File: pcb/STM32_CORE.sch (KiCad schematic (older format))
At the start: 31 parts, among them J6 Conn_01x14, J7 Conn_01x12, J8 Conn_01x12, SW1 SW_Push, U3 STM32F103C8T6, U4 AMS1117-3.3, Y1 O8M, Y2 O32.768K

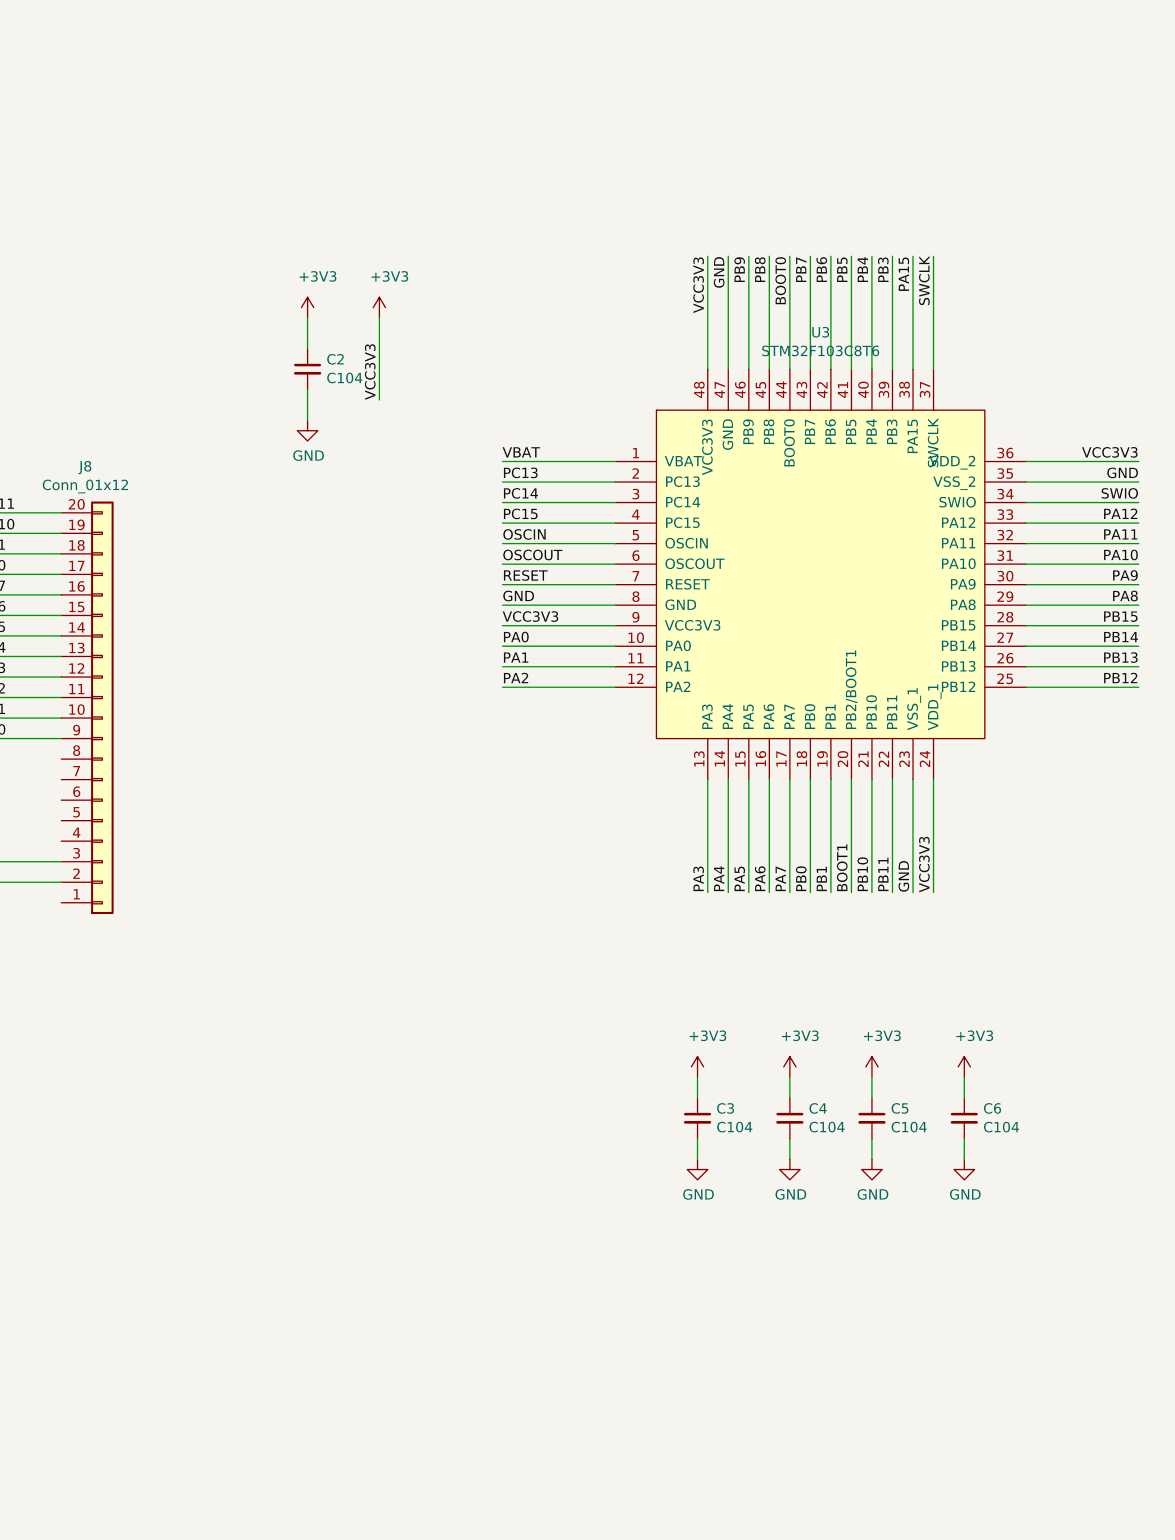
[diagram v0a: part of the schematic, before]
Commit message: update,
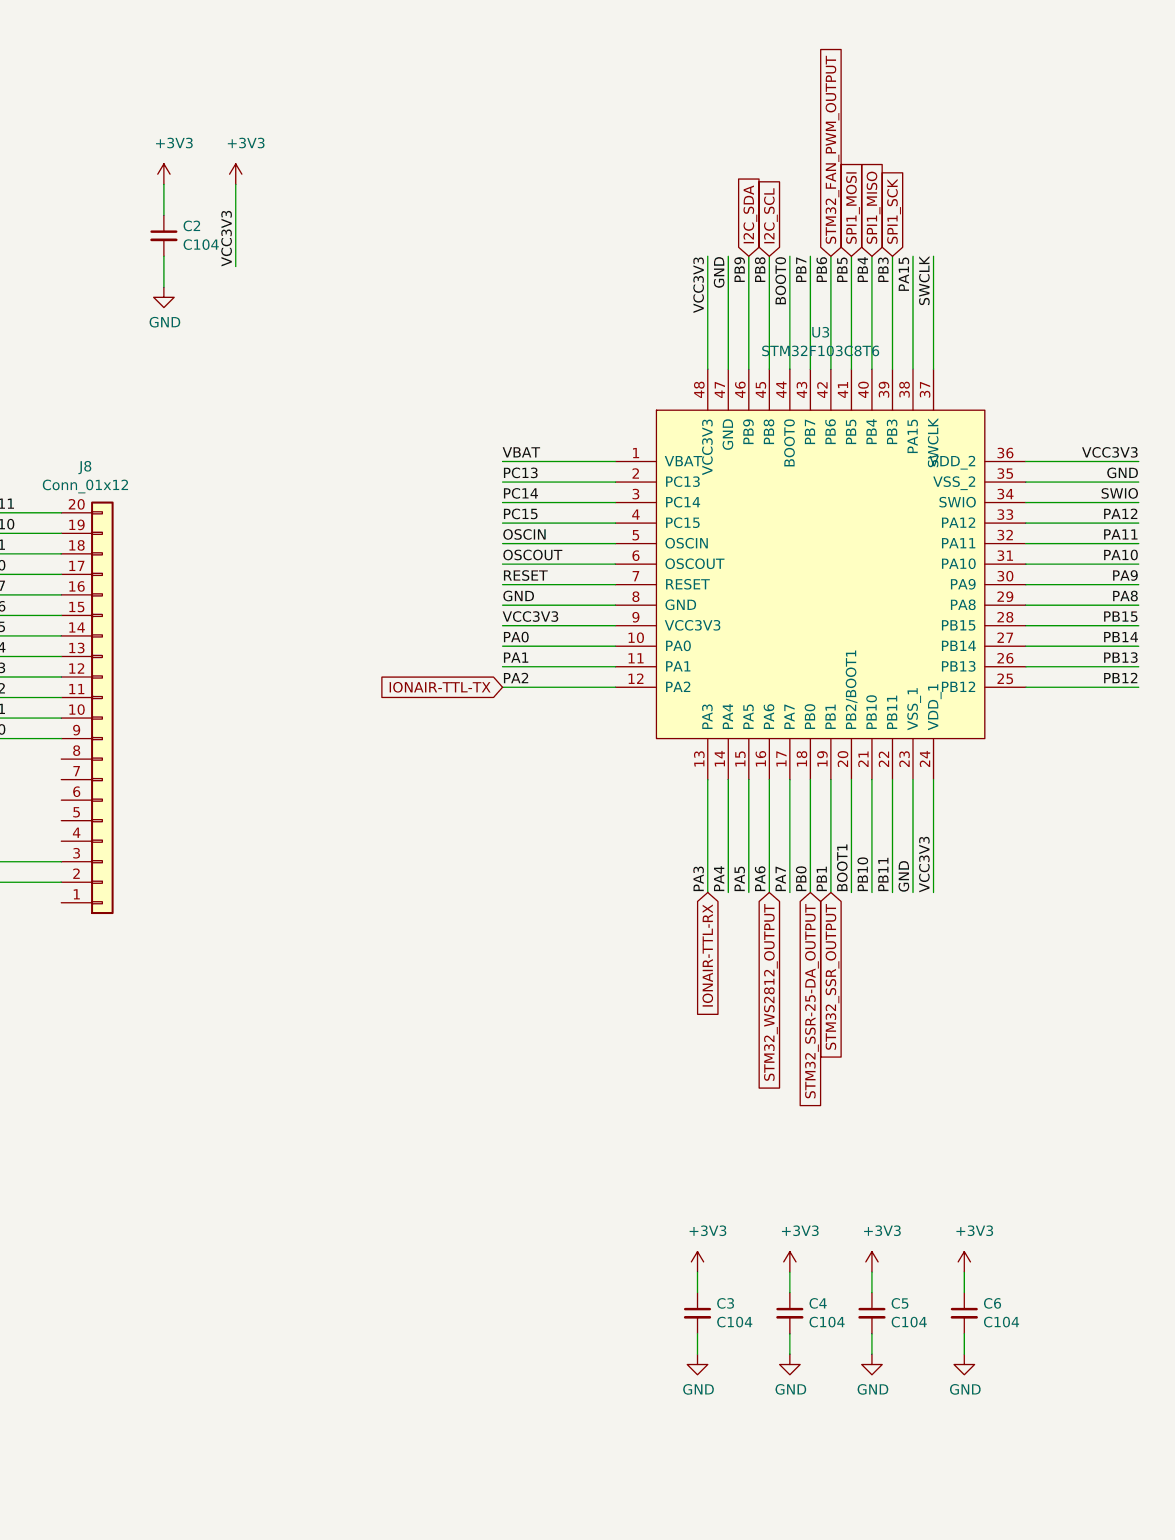
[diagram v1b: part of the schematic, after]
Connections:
- net PA2 renamed IONAIR-TTL-TX
- net PA3 renamed IONAIR-TTL-RX
- net PA6 renamed STM32_WS2812_OUTPUT
- net PB0 renamed STM32_SSR-25-DA_OUTPUT
- net PB1 renamed STM32_SSR_OUTPUT
- net PB3 renamed SPI1_SCK
- net PB4 renamed SPI1_MISO
- net PB5 renamed SPI1_MOSI
- net PB6 renamed STM32_FAN_PWM_OUTPUT
- net PB8 renamed I2C_SCL
- net PB9 renamed I2C_SDA
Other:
- moved on the sheet: C2, C3, C4, C5, C6
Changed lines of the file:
@@
 L taobao-c:C104 C3
 U 1 1 5BCBC4D6
-P 7850 5850
-F 0 "C3" H 7942 5896 50  0000 L CNN
-F 1 "C104" H 7942 5805 50  0000 L CNN
-F 2 "Capacitor_SMD:C_0603_1608Metric_Pad1.05x0.95mm_HandSolder" H 7850 5850 50  0001 C CNN
-F 3 "~" H 7850 5850 50  0001 C CNN
-	1    7850 5850
-	1    0    0    -1
-$EndComp
-Wire Wire Line
-	7850 5650 7850 5750
+P 7850 6800
+F 0 "C3" H 7942 6846 50  0000 L CNN
+F 1 "C104" H 7942 6755 50  0000 L CNN
+F 2 "Capacitor_SMD:C_0603_1608Metric_Pad1.05x0.95mm_HandSolder" H 7850 6800 50  0001 C CNN
+F 3 "~" H 7850 6800 50  0001 C CNN
+	1    7850 6800
+	1    0    0    -1
+$EndComp
+Wire Wire Line
+	7850 6600 7850 6700
 $Comp
 L power:GND #PWR026
 U 1 1 5BCBCE91
-P 7850 6050
-F 0 "#PWR026" H 7850 5800 50  0001 C CNN
-F 1 "GND" H 7855 5877 50  0000 C CNN
-F 2 "" H 7850 6050 50  0001 C CNN
-F 3 "" H 7850 6050 50  0001 C CNN
-	1    7850 6050
-	1    0    0    -1
-$EndComp
-Wire Wire Line
-	7850 5950 7850 6050
+P 7850 7000
+F 0 "#PWR026" H 7850 6750 50  0001 C CNN
+F 1 "GND" H 7855 6827 50  0000 C CNN
+F 2 "" H 7850 7000 50  0001 C CNN
+F 3 "" H 7850 7000 50  0001 C CNN
+	1    7850 7000
+	1    0    0    -1
+$EndComp
+Wire Wire Line
+	7850 6900 7850 7000
 $Comp
 L taobao-c:C104 C4
 U 1 1 5BCBD860
-P 8300 5850
-F 0 "C4" H 8392 5896 50  0000 L CNN
-F 1 "C104" H 8392 5805 50  0000 L CNN
-F 2 "Capacitor_SMD:C_0603_1608Metric_Pad1.05x0.95mm_HandSolder" H 8300 5850 50  0001 C CNN
-F 3 "~" H 8300 5850 50  0001 C CNN
-	1    8300 5850
-	1    0    0    -1
-$EndComp
-Wire Wire Line
-	8300 5650 8300 5750
+P 8300 6800
+F 0 "C4" H 8392 6846 50  0000 L CNN
+F 1 "C104" H 8392 6755 50  0000 L CNN
+F 2 "Capacitor_SMD:C_0603_1608Metric_Pad1.05x0.95mm_HandSolder" H 8300 6800 50  0001 C CNN
+F 3 "~" H 8300 6800 50  0001 C CNN
+	1    8300 6800
+	1    0    0    -1
+$EndComp
+Wire Wire Line
+	8300 6600 8300 6700
 $Comp
 L power:GND #PWR028
 U 1 1 5BCBD867
-P 8300 6050
-F 0 "#PWR028" H 8300 5800 50  0001 C CNN
-F 1 "GND" H 8305 5877 50  0000 C CNN
-F 2 "" H 8300 6050 50  0001 C CNN
-F 3 "" H 8300 6050 50  0001 C CNN
-	1    8300 6050
-	1    0    0    -1
-$EndComp
-Wire Wire Line
-	8300 5950 8300 6050
+P 8300 7000
+F 0 "#PWR028" H 8300 6750 50  0001 C CNN
+F 1 "GND" H 8305 6827 50  0000 C CNN
+F 2 "" H 8300 7000 50  0001 C CNN
+F 3 "" H 8300 7000 50  0001 C CNN
+	1    8300 7000
+	1    0    0    -1
+$EndComp
+Wire Wire Line
+	8300 6900 8300 7000
 $Comp
 L taobao-c:C104 C5
 U 1 1 5BCBE2F2
-P 8700 5850
-F 0 "C5" H 8792 5896 50  0000 L CNN
-F 1 "C104" H 8792 5805 50  0000 L CNN
-F 2 "Capacitor_SMD:C_0603_1608Metric_Pad1.05x0.95mm_HandSolder" H 8700 5850 50  0001 C CNN
-F 3 "~" H 8700 5850 50  0001 C CNN
-	1    8700 5850
-	1    0    0    -1
-$EndComp
-Wire Wire Line
-	8700 5650 8700 5750
+P 8700 6800
+F 0 "C5" H 8792 6846 50  0000 L CNN
+F 1 "C104" H 8792 6755 50  0000 L CNN
+F 2 "Capacitor_SMD:C_0603_1608Metric_Pad1.05x0.95mm_HandSolder" H 8700 6800 50  0001 C CNN
+F 3 "~" H 8700 6800 50  0001 C CNN
+	1    8700 6800
+	1    0    0    -1
+$EndComp
+Wire Wire Line
+	8700 6600 8700 6700
 $Comp
 L power:GND #PWR030
 U 1 1 5BCBE2F9
-P 8700 6050
-F 0 "#PWR030" H 8700 5800 50  0001 C CNN
-F 1 "GND" H 8705 5877 50  0000 C CNN
-F 2 "" H 8700 6050 50  0001 C CNN
-F 3 "" H 8700 6050 50  0001 C CNN
-	1    8700 6050
-	1    0    0    -1
-$EndComp
-Wire Wire Line
-	8700 5950 8700 6050
+P 8700 7000
+F 0 "#PWR030" H 8700 6750 50  0001 C CNN
+F 1 "GND" H 8705 6827 50  0000 C CNN
+F 2 "" H 8700 7000 50  0001 C CNN
+F 3 "" H 8700 7000 50  0001 C CNN
+	1    8700 7000
+	1    0    0    -1
+$EndComp
+Wire Wire Line
+	8700 6900 8700 7000
 $Comp
 L taobao-c:C104 C6
 U 1 1 5BCBE306
-P 9150 5850
-F 0 "C6" H 9242 5896 50  0000 L CNN
-F 1 "C104" H 9242 5805 50  0000 L CNN
-F 2 "Capacitor_SMD:C_0603_1608Metric_Pad1.05x0.95mm_HandSolder" H 9150 5850 50  0001 C CNN
-F 3 "~" H 9150 5850 50  0001 C CNN
-	1    9150 5850
-	1    0    0    -1
-$EndComp
-Wire Wire Line
-	9150 5650 9150 5750
+P 9150 6800
+F 0 "C6" H 9242 6846 50  0000 L CNN
+F 1 "C104" H 9242 6755 50  0000 L CNN
+F 2 "Capacitor_SMD:C_0603_1608Metric_Pad1.05x0.95mm_HandSolder" H 9150 6800 50  0001 C CNN
+F 3 "~" H 9150 6800 50  0001 C CNN
+	1    9150 6800
+	1    0    0    -1
+$EndComp
+Wire Wire Line
+	9150 6600 9150 6700
 $Comp
 L power:GND #PWR032
 U 1 1 5BCBE30D
-P 9150 6050
-F 0 "#PWR032" H 9150 5800 50  0001 C CNN
-F 1 "GND" H 9155 5877 50  0000 C CNN
-F 2 "" H 9150 6050 50  0001 C CNN
-F 3 "" H 9150 6050 50  0001 C CNN
-	1    9150 6050
-	1    0    0    -1
-$EndComp
-Wire Wire Line
-	9150 5950 9150 6050
+P 9150 7000
+F 0 "#PWR032" H 9150 6750 50  0001 C CNN
+F 1 "GND" H 9155 6827 50  0000 C CNN
+F 2 "" H 9150 7000 50  0001 C CNN
+F 3 "" H 9150 7000 50  0001 C CNN
+	1    9150 7000
+	1    0    0    -1
+$EndComp
+Wire Wire Line
+	9150 6900 9150 7000
 $Comp
 L taobao-osc:O32.768K Y2
@@
 L taobao-c:C104 C2
 U 1 1 5BD956B7
-P 5950 2200
-F 0 "C2" H 6042 2246 50  0000 L CNN
-F 1 "C104" H 6042 2155 50  0000 L CNN
-F 2 "Capacitor_SMD:C_0603_1608Metric_Pad1.05x0.95mm_HandSolder" H 5950 2200 50  0001 C CNN
-F 3 "~" H 5950 2200 50  0001 C CNN
-F 4 "near SWD" H 5950 2200 50  0001 C CNN "Field4"
-	1    5950 2200
+P 5250 1550
+F 0 "C2" H 5342 1596 50  0000 L CNN
+F 1 "C104" H 5342 1505 50  0000 L CNN
+F 2 "Capacitor_SMD:C_0603_1608Metric_Pad1.05x0.95mm_HandSolder" H 5250 1550 50  0001 C CNN
+F 3 "~" H 5250 1550 50  0001 C CNN
+F 4 "near SWD" H 5250 1550 50  0001 C CNN "Field4"
+	1    5250 1550
 	1    0    0    -1
 $EndComp
@@
 L power:GND #PWR023
 U 1 1 5BD957D4
-P 5950 2450
-F 0 "#PWR023" H 5950 2200 50  0001 C CNN
-F 1 "GND" H 5955 2277 50  0000 C CNN
-F 2 "" H 5950 2450 50  0001 C CNN
-F 3 "" H 5950 2450 50  0001 C CNN
-	1    5950 2450
-	1    0    0    -1
-$EndComp
-Wire Wire Line
-	5950 2300 5950 2450
-Wire Wire Line
-	5950 1950 5950 2100
+P 5250 1800
+F 0 "#PWR023" H 5250 1550 50  0001 C CNN
+F 1 "GND" H 5255 1627 50  0000 C CNN
+F 2 "" H 5250 1800 50  0001 C CNN
+F 3 "" H 5250 1800 50  0001 C CNN
+	1    5250 1800
+	1    0    0    -1
+$EndComp
+Wire Wire Line
+	5250 1650 5250 1800
+Wire Wire Line
+	5250 1300 5250 1450
 Text Label 2350 2600 2    50   ~ 0
 SWIO
@@
 	1    0    0    1
 $EndComp
-Text Label 6300 2350 1    50   ~ 0
+Text Label 5600 1700 1    50   ~ 0
 VCC3V3
 Wire Wire Line
-	6300 1950 6300 2350
+	5600 1300 5600 1700
 $Comp
 L Device:Jumper_NO_Small JP1
@@
 L power:+3V3 #PWR024
 U 1 1 5BCAD5BF
-P 6300 1950
-F 0 "#PWR024" H 6300 1800 50  0001 C CNN
-F 1 "+3V3" H 6350 2150 50  0000 C CNN
-F 2 "" H 6300 1950 50  0001 C CNN
-F 3 "" H 6300 1950 50  0001 C CNN
-	1    6300 1950
+P 5600 1300
+F 0 "#PWR024" H 5600 1150 50  0001 C CNN
+F 1 "+3V3" H 5650 1500 50  0000 C CNN
+F 2 "" H 5600 1300 50  0001 C CNN
+F 3 "" H 5600 1300 50  0001 C CNN
+	1    5600 1300
 	1    0    0    -1
 $EndComp
@@
 L power:+3V3 #PWR025
 U 1 1 5BCBE3DE
-P 7850 5650
-F 0 "#PWR025" H 7850 5500 50  0001 C CNN
-F 1 "+3V3" H 7900 5850 50  0000 C CNN
-F 2 "" H 7850 5650 50  0001 C CNN
-F 3 "" H 7850 5650 50  0001 C CNN
-	1    7850 5650
+P 7850 6600
+F 0 "#PWR025" H 7850 6450 50  0001 C CNN
+F 1 "+3V3" H 7900 6800 50  0000 C CNN
+F 2 "" H 7850 6600 50  0001 C CNN
+F 3 "" H 7850 6600 50  0001 C CNN
+	1    7850 6600
 	1    0    0    -1
 $EndComp
@@
 L power:+3V3 #PWR027
 U 1 1 5BCE7C1D
-P 8300 5650
-F 0 "#PWR027" H 8300 5500 50  0001 C CNN
-F 1 "+3V3" H 8350 5850 50  0000 C CNN
-F 2 "" H 8300 5650 50  0001 C CNN
-F 3 "" H 8300 5650 50  0001 C CNN
-	1    8300 5650
+P 8300 6600
+F 0 "#PWR027" H 8300 6450 50  0001 C CNN
+F 1 "+3V3" H 8350 6800 50  0000 C CNN
+F 2 "" H 8300 6600 50  0001 C CNN
+F 3 "" H 8300 6600 50  0001 C CNN
+	1    8300 6600
 	1    0    0    -1
 $EndComp
@@
 L power:+3V3 #PWR029
 U 1 1 5BCE7C66
-P 8700 5650
-F 0 "#PWR029" H 8700 5500 50  0001 C CNN
-F 1 "+3V3" H 8750 5850 50  0000 C CNN
-F 2 "" H 8700 5650 50  0001 C CNN
-F 3 "" H 8700 5650 50  0001 C CNN
-	1    8700 5650
+P 8700 6600
+F 0 "#PWR029" H 8700 6450 50  0001 C CNN
+F 1 "+3V3" H 8750 6800 50  0000 C CNN
+F 2 "" H 8700 6600 50  0001 C CNN
+F 3 "" H 8700 6600 50  0001 C CNN
+	1    8700 6600
 	1    0    0    -1
 $EndComp
@@
 L power:+3V3 #PWR031
 U 1 1 5BCE7CAF
-P 9150 5650
-F 0 "#PWR031" H 9150 5500 50  0001 C CNN
-F 1 "+3V3" H 9200 5850 50  0000 C CNN
-F 2 "" H 9150 5650 50  0001 C CNN
-F 3 "" H 9150 5650 50  0001 C CNN
-	1    9150 5650
+P 9150 6600
+F 0 "#PWR031" H 9150 6450 50  0001 C CNN
+F 1 "+3V3" H 9200 6800 50  0000 C CNN
+F 2 "" H 9150 6600 50  0001 C CNN
+F 3 "" H 9150 6600 50  0001 C CNN
+	1    9150 6600
 	1    0    0    -1
 $EndComp
@@
 L power:+3V3 #PWR022
 U 1 1 5BCF284B
-P 5950 1950
-F 0 "#PWR022" H 5950 1800 50  0001 C CNN
-F 1 "+3V3" H 6000 2150 50  0000 C CNN
-F 2 "" H 5950 1950 50  0001 C CNN
-F 3 "" H 5950 1950 50  0001 C CNN
-	1    5950 1950
+P 5250 1300
+F 0 "#PWR022" H 5250 1150 50  0001 C CNN
+F 1 "+3V3" H 5300 1500 50  0000 C CNN
+F 2 "" H 5250 1300 50  0001 C CNN
+F 3 "" H 5250 1300 50  0001 C CNN
+	1    5250 1300
 	1    0    0    -1
 $EndComp
@@
 	0    -1   -1   0
 $EndComp
+Text GLabel 8100 1650 1    50   Input ~ 0
+I2C_SDA
+Text GLabel 8200 1650 1    50   Input ~ 0
+I2C_SCL
+Text GLabel 8600 1650 1    50   Input ~ 0
+SPI1_MOSI
+Text GLabel 8700 1650 1    50   Input ~ 0
+SPI1_MISO
+Text GLabel 8800 1650 1    50   Input ~ 0
+SPI1_SCK
+Text GLabel 8500 1650 1    50   Input ~ 0
+STM32_FAN_PWM_OUTPUT
+Text GLabel 8500 4750 3    50   Input ~ 0
+STM32_SSR_OUTPUT
+Text GLabel 8400 4750 3    50   Input ~ 0
+STM32_SSR-25-DA_OUTPUT
+Text GLabel 6900 3750 0    50   Input ~ 0
+IONAIR-TTL-TX
+Text GLabel 7900 4750 3    50   Input ~ 0
+IONAIR-TTL-RX
+Text GLabel 8200 4750 3    50   Input ~ 0
+STM32_WS2812_OUTPUT
 $EndSCHEMATC
